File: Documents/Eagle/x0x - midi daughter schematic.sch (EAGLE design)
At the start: 8 parts

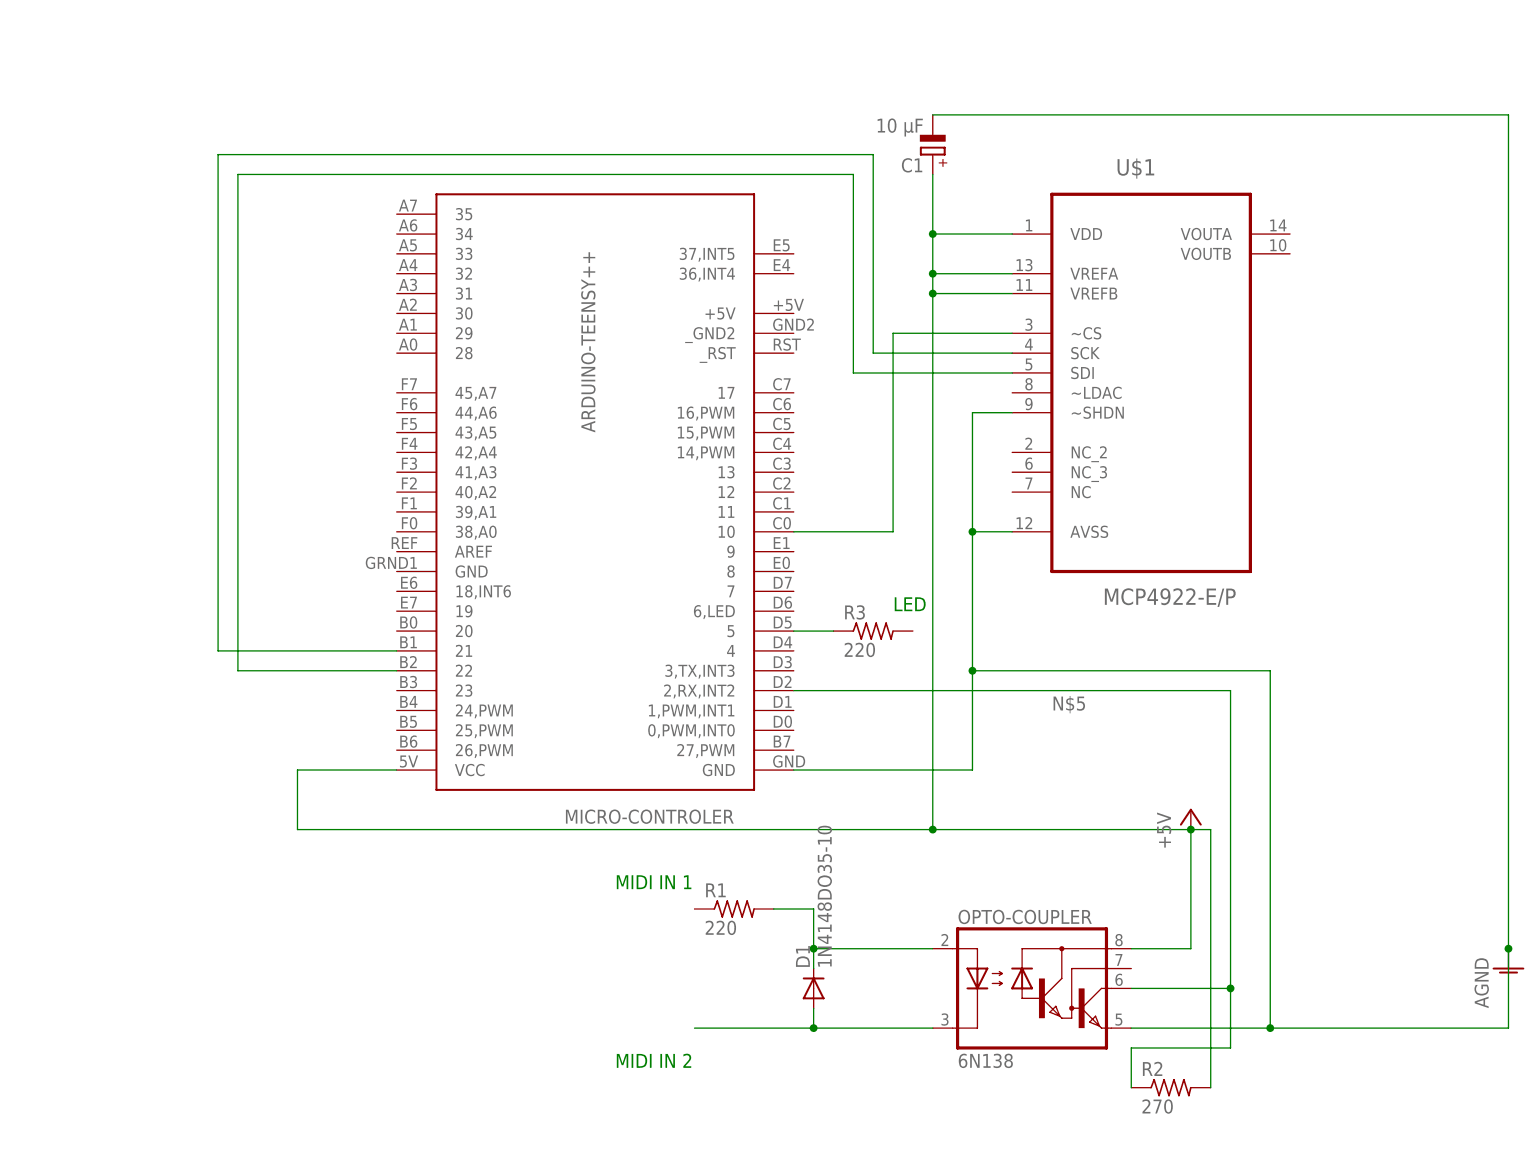
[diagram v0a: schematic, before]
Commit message: Finalise PCB
Finish PCB v 1.0
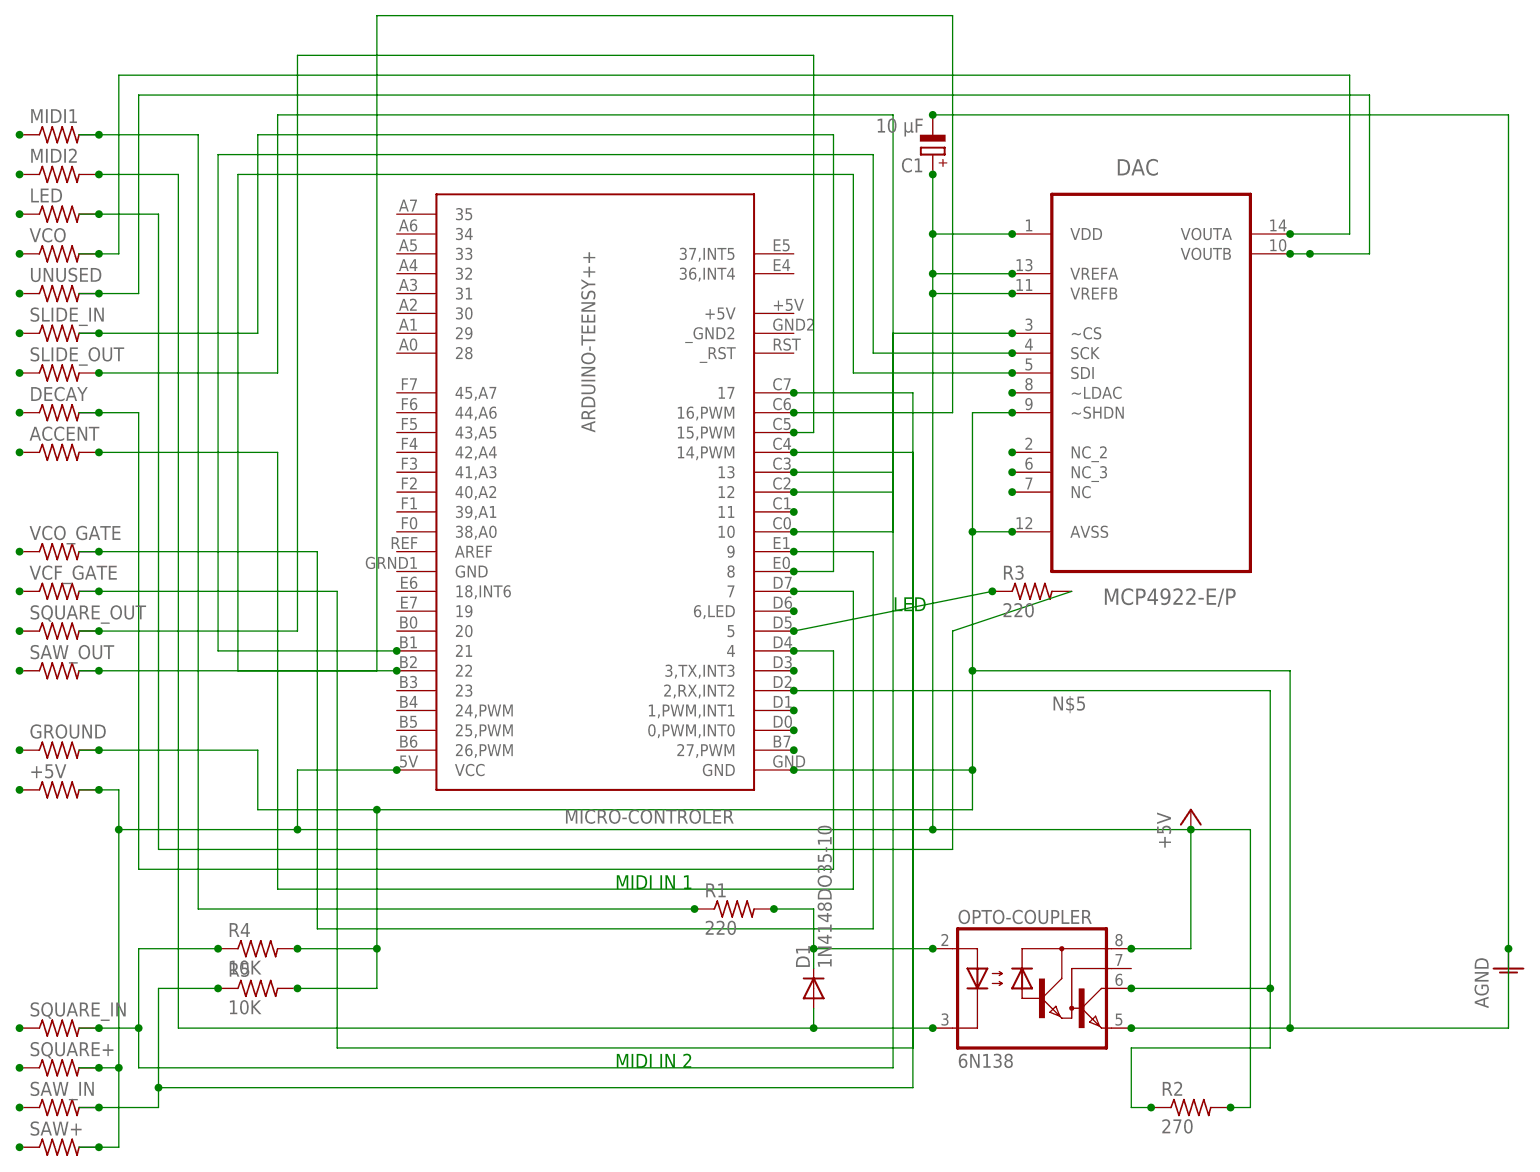
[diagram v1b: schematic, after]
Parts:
- added +5V, ACCENT, DECAY, GROUND, LED, MIDI1, MIDI2, SAW+, SAW_IN, SAW_OUT, SLIDE_IN, SLIDE_OUT, SQUARE+, SQUARE_IN, SQUARE_OUT, UNUSED, VCF_GATE, VCO, VCO_GATE: (no value), rcl:R-US_0207/10
- added R4, R5: 10K, rcl:R-US_0207/10
- renumbered U$1 to DAC
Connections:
- new net N$10: LED.2, R3.2
- new net N$11: DAC.VOUTA, VCO.2
- new net N$12: DAC.VOUTB, UNUSED.2
- new net N$13: MICRO-CONTROLER.8, SLIDE_IN.2
- new net N$14: DECAY.2, MICRO-CONTROLER.4
- new net N$15: ACCENT.2, MICRO-CONTROLER.7
- new net N$16: MICRO-CONTROLER.9, VCO_GATE.2
- new net N$17: MICRO-CONTROLER.17, VCF_GATE.2
- new net N$18: MICRO-CONTROLER.13, R4.1, SQUARE_IN.2
- new net N$19: MICRO-CONTROLER.14,PWM, R5.1, SAW_IN.2
- new net N$20: SAW+.1
- new net N$21: SAW_IN.1
- new net N$22: SQUARE+.1
- new net N$23: MICRO-CONTROLER.15,PWM, SQUARE_OUT.2
- new net N$24: MICRO-CONTROLER.16,PWM, SAW_OUT.2
- new net N$25: SQUARE_IN.1
- new net N$26: +5V.1
- new net N$27: GROUND.1
- new net N$28: SAW_OUT.1
- new net N$29: SQUARE_OUT.1
- new net N$30: VCF_GATE.1
- new net N$31: VCO_GATE.1
- new net N$32: ACCENT.1
- new net N$33: DECAY.1
- new net N$34: SLIDE_OUT.1
- new net N$35: SLIDE_IN.1
- new net N$36: UNUSED.1
- new net N$37: VCO.1
- new net N$38: LED.1
- new net N$39: MIDI2.1
- new net N$40: MIDI1.1
- new net N$41: DAC.~LDAC
- new net N$42: DAC.NC_2
- new net N$43: DAC.NC_3
- new net N$44: DAC.NC
- new net N$45: MICRO-CONTROLER.11
- new net N$46: MICRO-CONTROLER.6,LED
- new net N$47: MICRO-CONTROLER.3,TX,INT3
- new net N$48: MICRO-CONTROLER.1,PWM,INT1
- new net N$49: MICRO-CONTROLER.0,PWM,INT0
- new net N$50: MICRO-CONTROLER.27,PWM
- new net N$8: MIDI1.2, R1.1
- new net N$9: MICRO-CONTROLER.12, SLIDE_OUT.2
- net +5V: now also +5V.2, SAW+.2, SQUARE+.2
- net AGND: now also GROUND.2, R4.2, R5.2
- net N$4: now also MIDI2.2
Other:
- moved on the sheet: R2, R3
